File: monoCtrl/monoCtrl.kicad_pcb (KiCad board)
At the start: 2 copper layers, 48.3 x 83.8 mm, 15 parts, among them J1 Conn_01x08_Pin, J2 Conn_01x08_Pin, J3 Conn_01x08_Pin, J4 Conn_01x08_Pin, J5 Conn_01x08_Pin, J6 Jack-DC

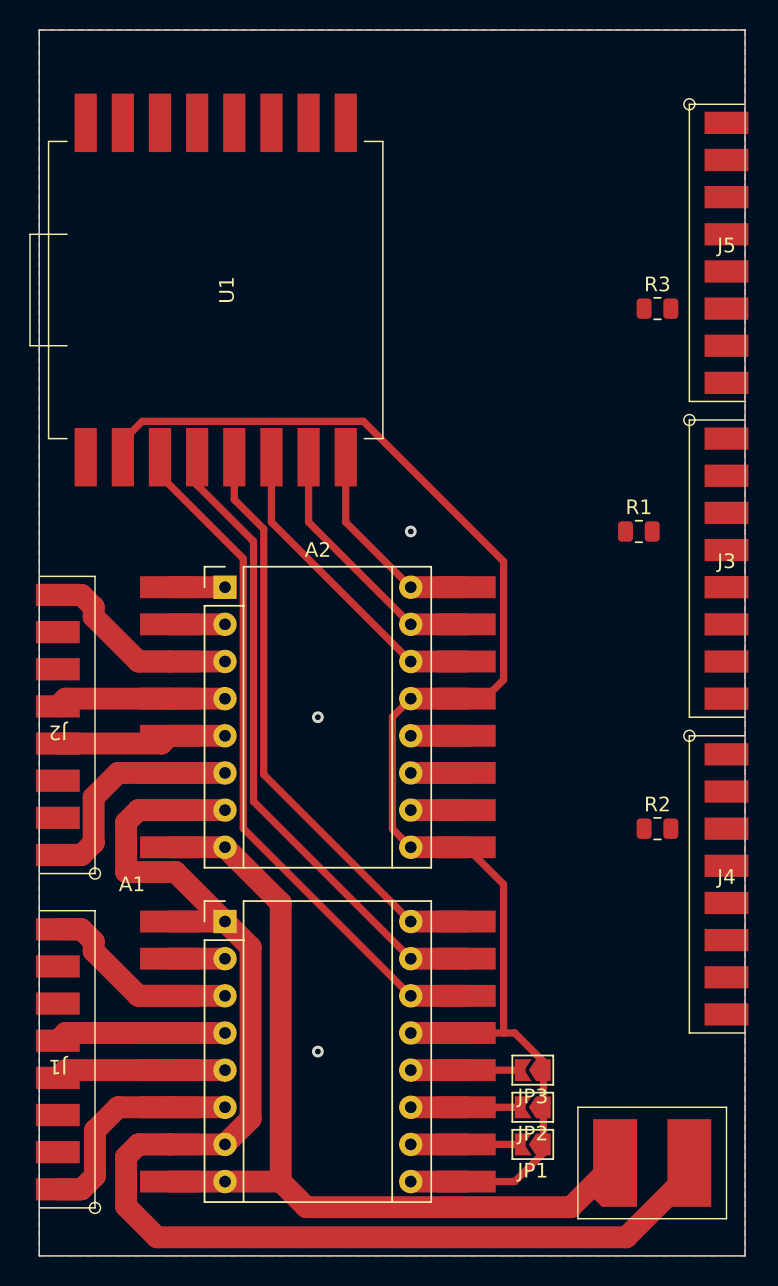
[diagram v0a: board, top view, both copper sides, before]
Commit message: finished v0.1
ready to etch
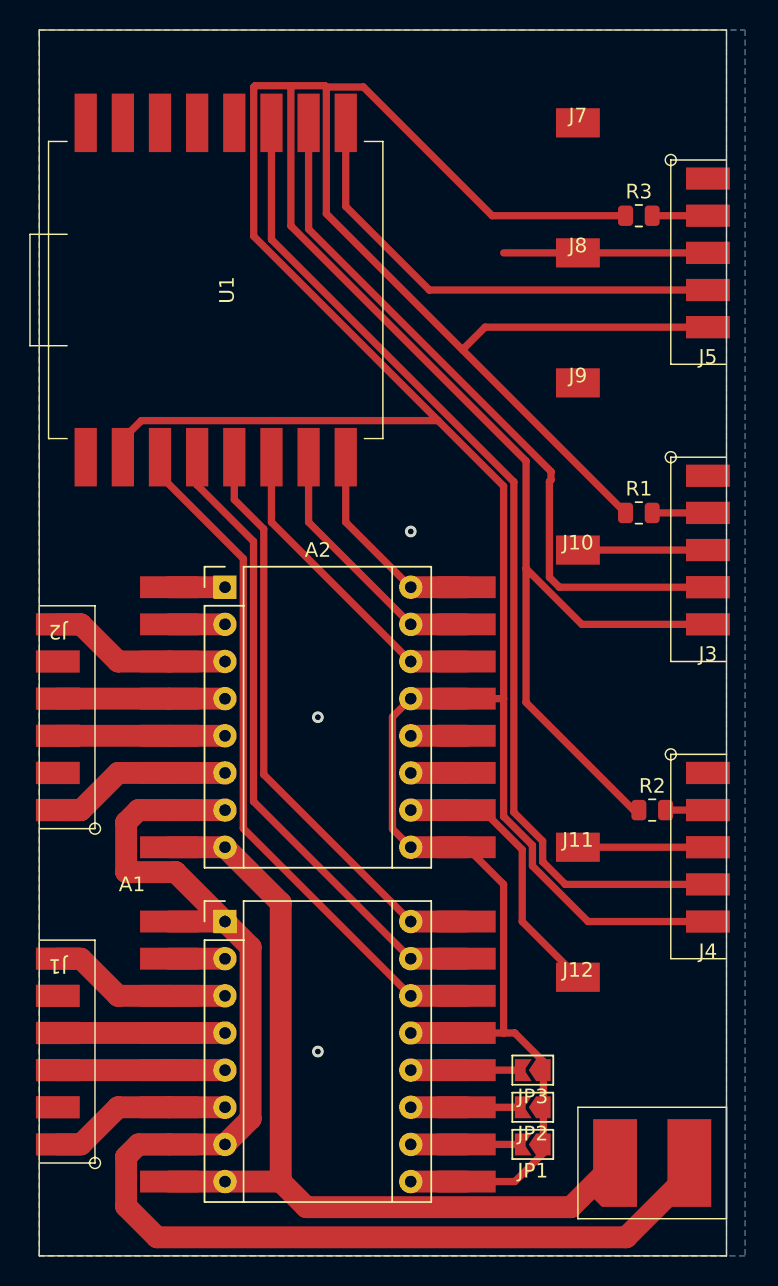
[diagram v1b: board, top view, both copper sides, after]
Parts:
- added J10: Conn_01x01_Pin, uC:air jump, F.Cu at (88.9, 109.2)
- added J11: Conn_01x01_Pin, uC:air jump, F.Cu at (88.9, 129.5)
- added J12: Conn_01x01_Pin, uC:air jump, F.Cu at (88.9, 138.4)
- added J7: Conn_01x01_Pin, uC:air jump, F.Cu at (88.9, 80.0)
- added J8: Conn_01x01_Pin, uC:air jump, F.Cu at (88.9, 88.9)
- added J9: Conn_01x01_Pin, uC:air jump, F.Cu at (88.9, 97.8)
- J1, J2: value Conn_01x08_Pin -> Conn_01x06_Pin; footprint uC:1x08_BoardEdge -> uC:1x06_BoardEdge
- J3, J4, J5: value Conn_01x08_Pin -> Conn_01x05_Pin; footprint uC:1x08_BoardEdge -> uC:1x05_BoardEdge
- moved R3 6.48 mm to (93.1, 86.4)
- moved J4 2.84 mm to (97.8, 129.5)
- moved J2 1.80 mm to (53.3, 119.4)
- moved J1 1.80 mm to (53.3, 142.2)
- moved J3 1.80 mm to (97.8, 109.2)
- moved R2 1.32 mm to (94.0, 127.0)
- moved J5 1.27 mm to (97.8, 88.9)
- moved R1 1.27 mm to (93.1, 106.7)
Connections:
- J1 pad 3: unconnected-(J1-Pin_3-Pad3) -> Net-(A1-B1)
- J1 pad 4: Net-(A1-B1) -> Net-(A1-A1)
- J1 pad 5: Net-(A1-A1) -> unconnected-(J1-Pin_5-Pad5)
- J1 pad 6: unconnected-(J1-Pin_6-Pad6) -> Net-(A1-A2)
- J2 pad 3: unconnected-(J2-Pin_3-Pad3) -> Net-(A2-B1)
- J2 pad 4: Net-(A2-B1) -> Net-(A2-A1)
- J2 pad 5: Net-(A2-A1) -> unconnected-(J2-Pin_5-Pad5)
- J2 pad 6: unconnected-(J2-Pin_6-Pad6) -> Net-(A2-A2)
- J3 pad 1: unconnected-(J3-Pin_1-Pad1) -> GND
- J3 pad 2: unconnected-(J3-Pin_2-Pad2) -> /StallDetectLED
- J3 pad 3: unconnected-(J3-Pin_3-Pad3) -> GND
- J3 pad 4: GND -> /StallDetect
- J3 pad 5: /StallDetectLED -> +5V
- J4 pad 1: unconnected-(J4-Pin_1-Pad1) -> GND
- J4 pad 2: unconnected-(J4-Pin_2-Pad2) -> /ZeroDetectLED
- J4 pad 3: unconnected-(J4-Pin_3-Pad3) -> GND
- J4 pad 4: GND -> /ZeroDetect
- J4 pad 5: /ZeroDetect -> +5V
- J5 pad 1: unconnected-(J5-Pin_1-Pad1) -> GND
- J5 pad 2: unconnected-(J5-Pin_2-Pad2) -> /GratingDetectLED
- J5 pad 3: unconnected-(J5-Pin_3-Pad3) -> GND
- J5 pad 4: GND -> /GratingDetect
- J5 pad 5: /GratingDetect -> +5V
- U1 pad 10: unconnected-(U1-SCL/D3-Pad10) -> /StallDetect
- U1 pad 11: /GratingDetect -> /ZeroDetect
- U1 pad 12: /ZeroDetect -> unconnected-(U1-TX/D1-Pad12)
- U1 pad 13: /StallDetect -> unconnected-(U1-RX/D0-Pad13)
- U1 pad 9: unconnected-(U1-D9-Pad9) -> /GratingDetect
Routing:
- net +5V: track 101.4 -> 317.0 mm
- net /ZeroDetect: track 0.00 -> 70.1 mm
- net /StallDetect: track 0.00 -> 49.1 mm
- net GND: track 106.9 -> 153.8 mm
- net /GratingDetect: track 0.00 -> 32.8 mm
- net /StallDetectLED: track 0.00 -> 3.81 mm
- net /GratingDetectLED: track 0.00 -> 3.81 mm
- net Net-(A2-B2): track 15.6 -> 12.5 mm
- net Net-(A1-B2): track 15.6 -> 12.5 mm
- net /ZeroDetectLED: track 0.00 -> 2.90 mm
- net Net-(A2-A2): track 13.7 -> 12.5 mm
- net Net-(A1-A2): track 13.7 -> 12.5 mm
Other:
- board size 48.3 x 83.8 mm -> 47 x 83.8 mm
